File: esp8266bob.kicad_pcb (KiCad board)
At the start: 2 copper layers, 50 x 50 mm, 46 parts, among them P1 USB_OTG, P2 CONN_01X07, P3 CONN_01X07, P4 CONN_01X03, U1 TS 2940 CP33, U10 WS2812, U11 WS2812, U12 WS2812, U2 ESP-07v2, U3 WS2812, U4 WS2812, U5 WS2812, U6 WS2812, U7 WS2812, U8 WS2812, U9 CH340G, Y1 12M

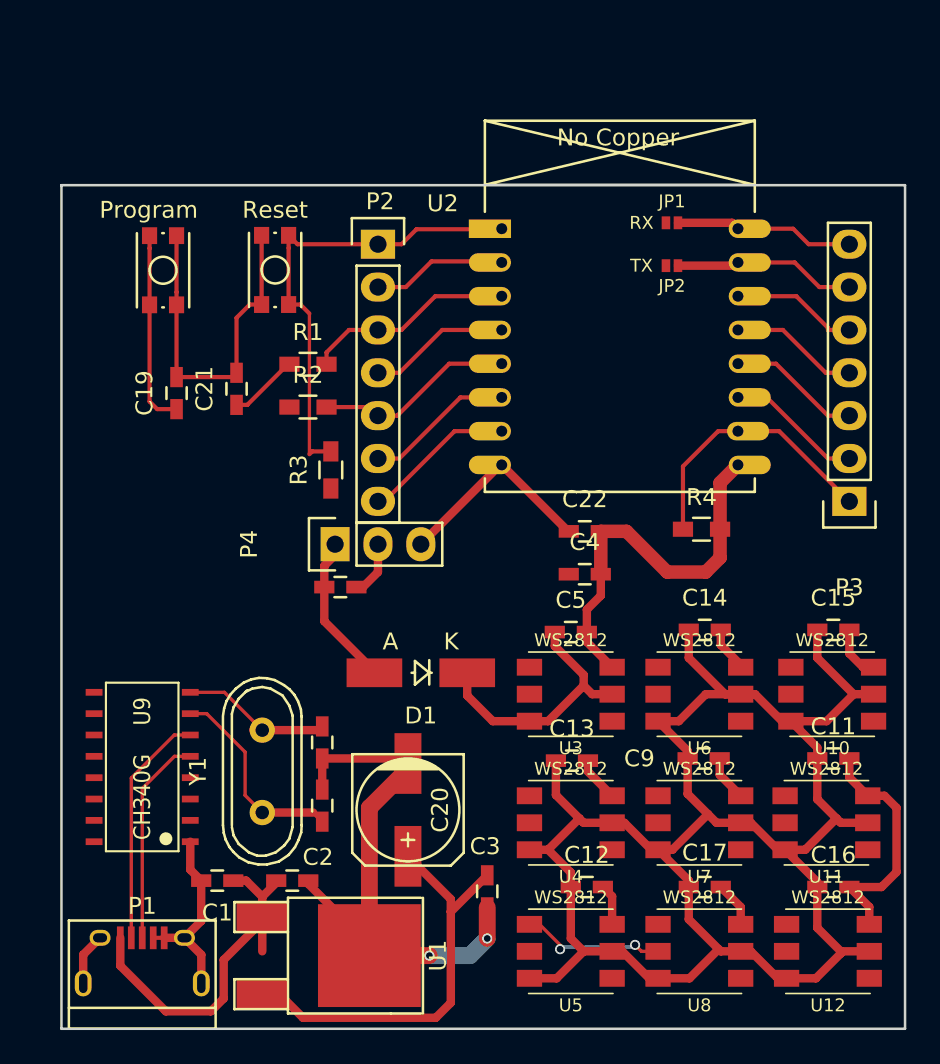
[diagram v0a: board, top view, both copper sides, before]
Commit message: PCB!!!
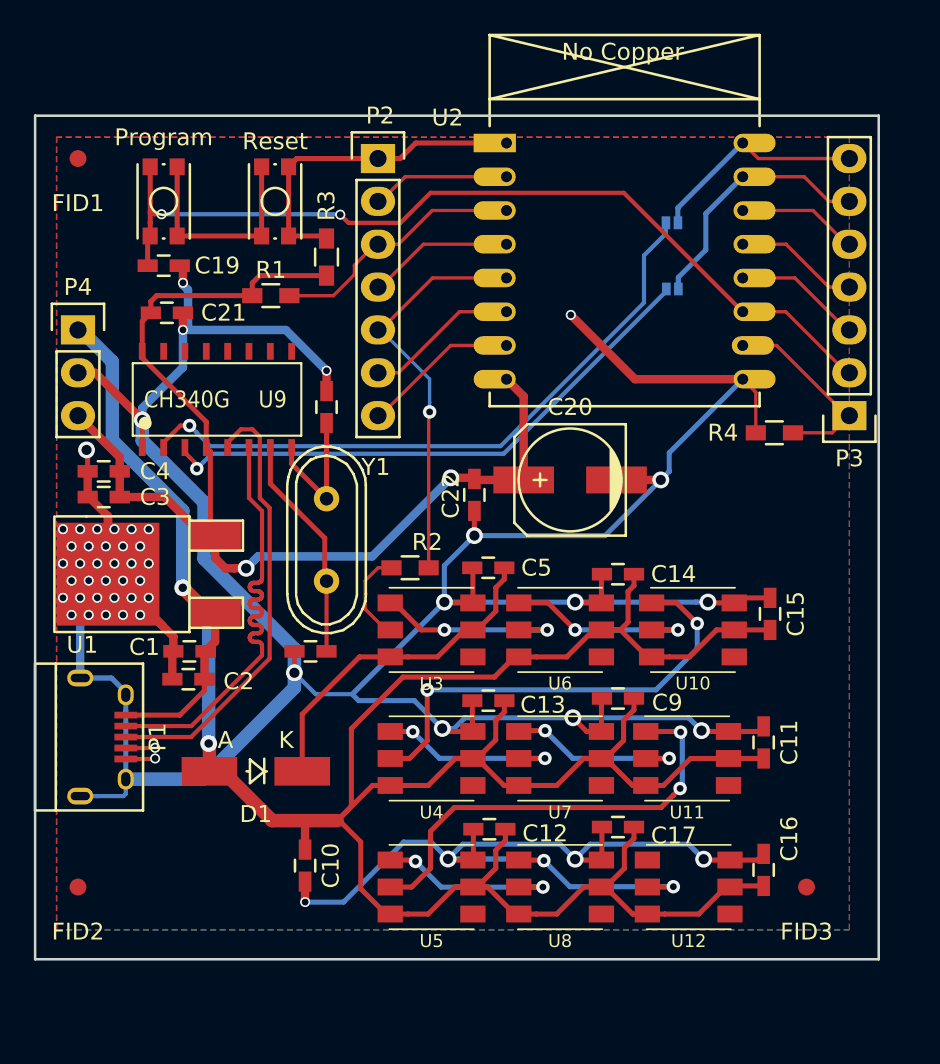
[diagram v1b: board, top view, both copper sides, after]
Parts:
- added FID1: Fiducial_1mm_Dia_2.54mm_Outer_CopperTop, Fiducials:Fiducial_1mm_Dia_2.54mm_Outer_CopperTop, F.Cu at (221.0, 58.4)
- added FID2: Fiducial_1mm_Dia_2.54mm_Outer_CopperTop, Fiducials:Fiducial_1mm_Dia_2.54mm_Outer_CopperTop, F.Cu at (221.0, 101.6)
- added FID3: Fiducial_1mm_Dia_2.54mm_Outer_CopperTop, Fiducials:Fiducial_1mm_Dia_2.54mm_Outer_CopperTop, F.Cu at (264.2, 101.6)
- JP1, JP2: moved to B.Cu
- moved C3 32.6 mm to (222.5, 78.5), turned to 180 degrees
- moved C4 29.2 mm to (222.5, 77.0), turned to 180 degrees
- moved U1 22.8 mm to (229.1, 83.1), turned to 90 degrees
- moved U9 22.2 mm to (229.2, 72.7), turned to 0 degrees
- moved C20 21.8 mm to (250.1, 77.5), turned to 180 degrees
- moved C7 19.9 mm to (235.7, 73.2), turned to 270 degrees
- moved P4 19.8 mm to (221.0, 68.6), turned to 0 degrees
- moved C10 16.6 mm to (234.4, 100.3), turned to 270 degrees
- moved Y1 14.2 mm to (235.7, 81.0)
- moved P1 13.7 mm to (222.2, 92.7), turned to 270 degrees
- moved C1 13.7 mm to (227.6, 87.6)
- moved C2 13.4 mm to (227.5, 89.3), turned to 180 degrees
- moved R3 12.6 mm to (235.7, 64.3)
- moved D1 11.4 mm to (231.5, 94.7)
- moved R2 11.3 mm to (240.7, 82.7)
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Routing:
- net GND: track 127.8 -> 308.2 mm, vias 2 -> 54
- net (no net): track 106.0 -> 0.00 mm
- net /CH340_RX: track 0.00 -> 38.5 mm, vias 0 -> 1
- net /CH340_TX: track 0.00 -> 33.9 mm, vias 0 -> 1
- net /Prog_pin: track 19.7 -> 52.8 mm, vias 0 -> 2
- net +5V: track 142.8 -> 170.3 mm, vias 0 -> 2
- net Net-(U10-Pad1): track 0.00 -> 27.4 mm, vias 0 -> 2
- net +3V3: track 41.4 -> 68.4 mm, vias 0 -> 2
- net Net-(U11-Pad1): track 0.00 -> 26.4 mm, vias 0 -> 2
- net /USB_D+: track 12.5 -> 26.6 mm
- net /USB_D-: track 14.0 -> 26.6 mm
- net /GPIO14: track 11.9 -> 24.4 mm, vias 0 -> 1
- net Net-(U3-Pad1): track 0.00 -> 12.3 mm, vias 0 -> 2
- net Net-(U10-Pad2): track 0.00 -> 11.7 mm, vias 0 -> 2
- net Net-(U4-Pad1): track 0.00 -> 11.4 mm, vias 0 -> 2
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- added copper zone on B.Cu, net GND
- added copper zone on F.Cu, net GND
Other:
- net class Default: trace_width 0.1524 -> 0.2
- net class Power added: clearance 0.2, trace_width 0.5, via_dia 1, via_drill 0.6
- rule trace_min: 0.1524 -> 0.2
- rule via_min_size: 0.4 -> 0.6
